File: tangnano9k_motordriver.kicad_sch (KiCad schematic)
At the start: 43 parts, among them J1 Jack-DC, J2 Screw_Terminal_01x04, J3 Screw_Terminal_01x04, J4 Pmod, SW3 SW_DIP_x08, U1 BP5293-5, U2 TB67S101ANG, U3 TangNano9K, U4 OSL641505-BB, U5 TB67S101ANG

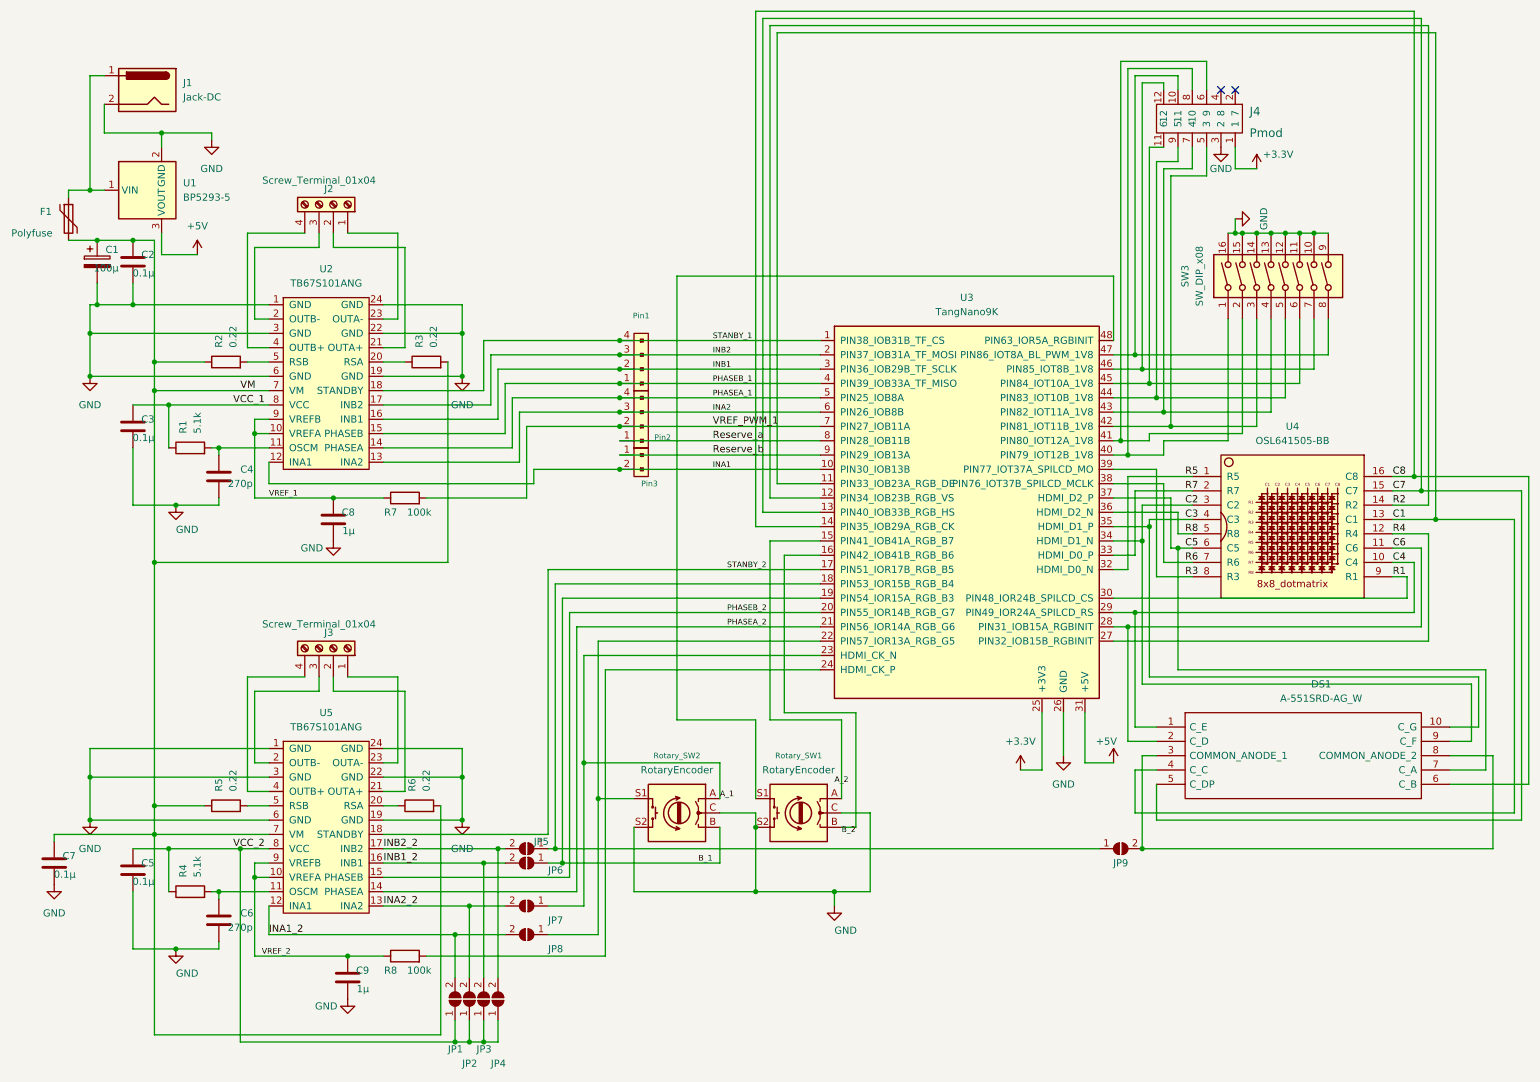
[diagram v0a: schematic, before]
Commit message: 17
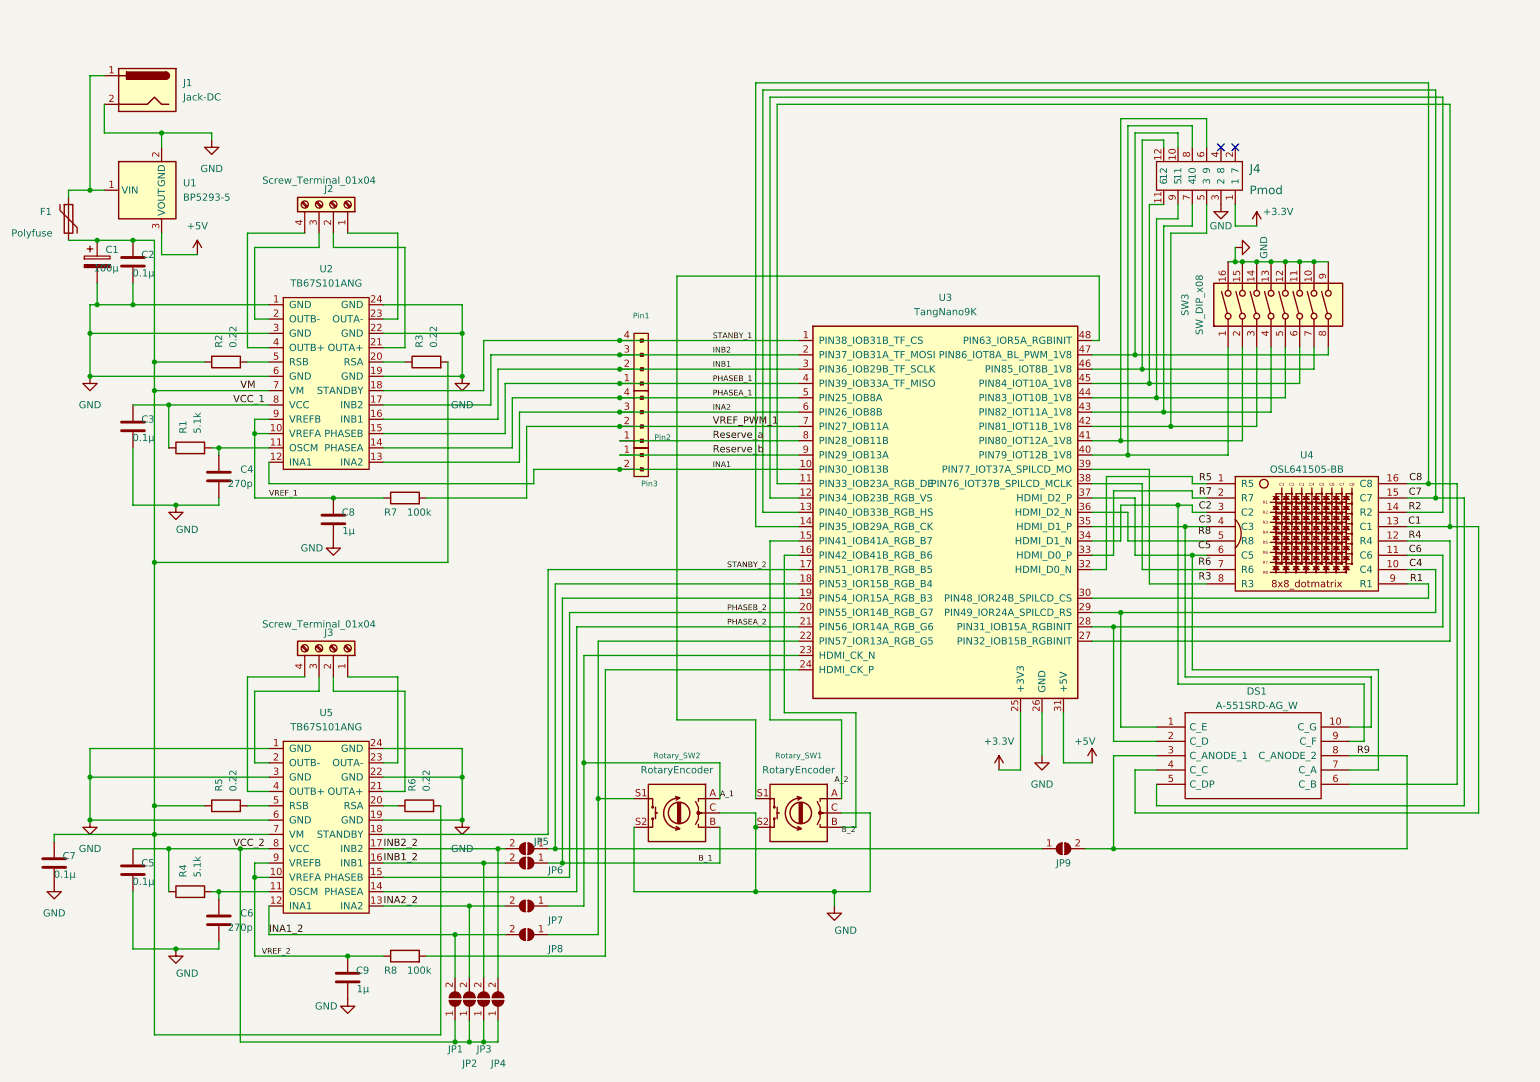
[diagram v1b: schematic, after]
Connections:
- net C1: no longer DS1.4 (C_C), U3.11 (PIN33_IOB23A_RGB_DE), U4.13 (C1)
- net C2: no longer DS1.9 (C_F), U3.34 (HDMI_D1_N), U4.3 (C2)
- net C3: no longer DS1.10 (C_G), U3.35 (HDMI_D1_P), U4.4 (C3)
- net C4: no longer DS1.1 (C_E), U3.29 (PIN49_IOR24A_SPILCD_RS), U4.10 (C4)
- net C5: no longer DS1.7 (C_A), U3.37 (HDMI_D2_P), U4.6 (C5)
- net C6: no longer DS1.2 (C_D), U3.28 (PIN31_IOB15A_RGBINIT), U4.11 (C6)
- net C7: no longer DS1.5 (C_DP), U3.13 (PIN40_IOB33B_RGB_HS), U4.15 (C7)
- net C8: no longer DS1.6 (C_B), U3.14 (PIN35_IOB29A_RGB_CK), U4.16 (C8)
- net R2: no longer U3.12 (PIN34_IOB23B_RGB_VS), U4.14 (R2)
- net R3: no longer U3.39 (PIN77_IOT37A_SPILCD_MO), U4.8 (R3)
- net R4: no longer U3.27 (PIN32_IOB15B_RGBINIT), U4.12 (R4)
- net R5: no longer U3.32 (HDMI_D0_N), U4.1 (R5)
- net R6: no longer U3.38 (PIN76_IOT37B_SPILCD_MCLK), U4.7 (R6)
- net R7: no longer U3.33 (HDMI_D0_P), U4.2 (R7)
- net R8: no longer U3.36 (HDMI_D2_N), U4.5 (R8)
- net R9: now reaches DS1.3 (C_ANODE_1), DS1.8 (C_ANODE_2), JP9.2 (B)
- new net: U3.32 (HDMI_D0_N), U4.1 (R5)
- new net: DS1.1 (C_E), U3.29 (PIN49_IOR24A_SPILCD_RS), U4.10 (C4)
- new net: DS1.2 (C_D), U3.28 (PIN31_IOB15A_RGBINIT), U4.11 (C6)
- new net: U3.27 (PIN32_IOB15B_RGBINIT), U4.12 (R4)
- new net: DS1.4 (C_C), U3.11 (PIN33_IOB23A_RGB_DE), U4.13 (C1)
- new net: U3.12 (PIN34_IOB23B_RGB_VS), U4.14 (R2)
- new net: DS1.5 (C_DP), U3.13 (PIN40_IOB33B_RGB_HS), U4.15 (C7)
- new net: DS1.6 (C_B), U3.14 (PIN35_IOB29A_RGB_CK), U4.16 (C8)
- new net: U3.33 (HDMI_D0_P), U4.2 (R7)
- new net: DS1.9 (C_F), U3.34 (HDMI_D1_N), U4.3 (C2)
- new net: DS1.10 (C_G), U3.35 (HDMI_D1_P), U4.4 (C3)
- new net: U3.36 (HDMI_D2_N), U4.5 (R8)
- new net: DS1.7 (C_A), U3.37 (HDMI_D2_P), U4.6 (C5)
- new net: U3.38 (PIN76_IOT37B_SPILCD_MCLK), U4.7 (R6)
- new net: U3.39 (PIN77_IOT37A_SPILCD_MO), U4.8 (R3)
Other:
- moved on the sheet: DS1, J4, JP9, SW3, U3, U4
